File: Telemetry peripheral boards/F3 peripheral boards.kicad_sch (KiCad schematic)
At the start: 37 parts, among them J1 ATS668LSM, J2 1053131108, J3 Potentiometer, J4 Strain Gauge, U1 LM2907M/NOPB, U2 INA125U, U3 MCP2515-I/SO, U4 ISO1050DUB, U5 ATTINY1616-MNR

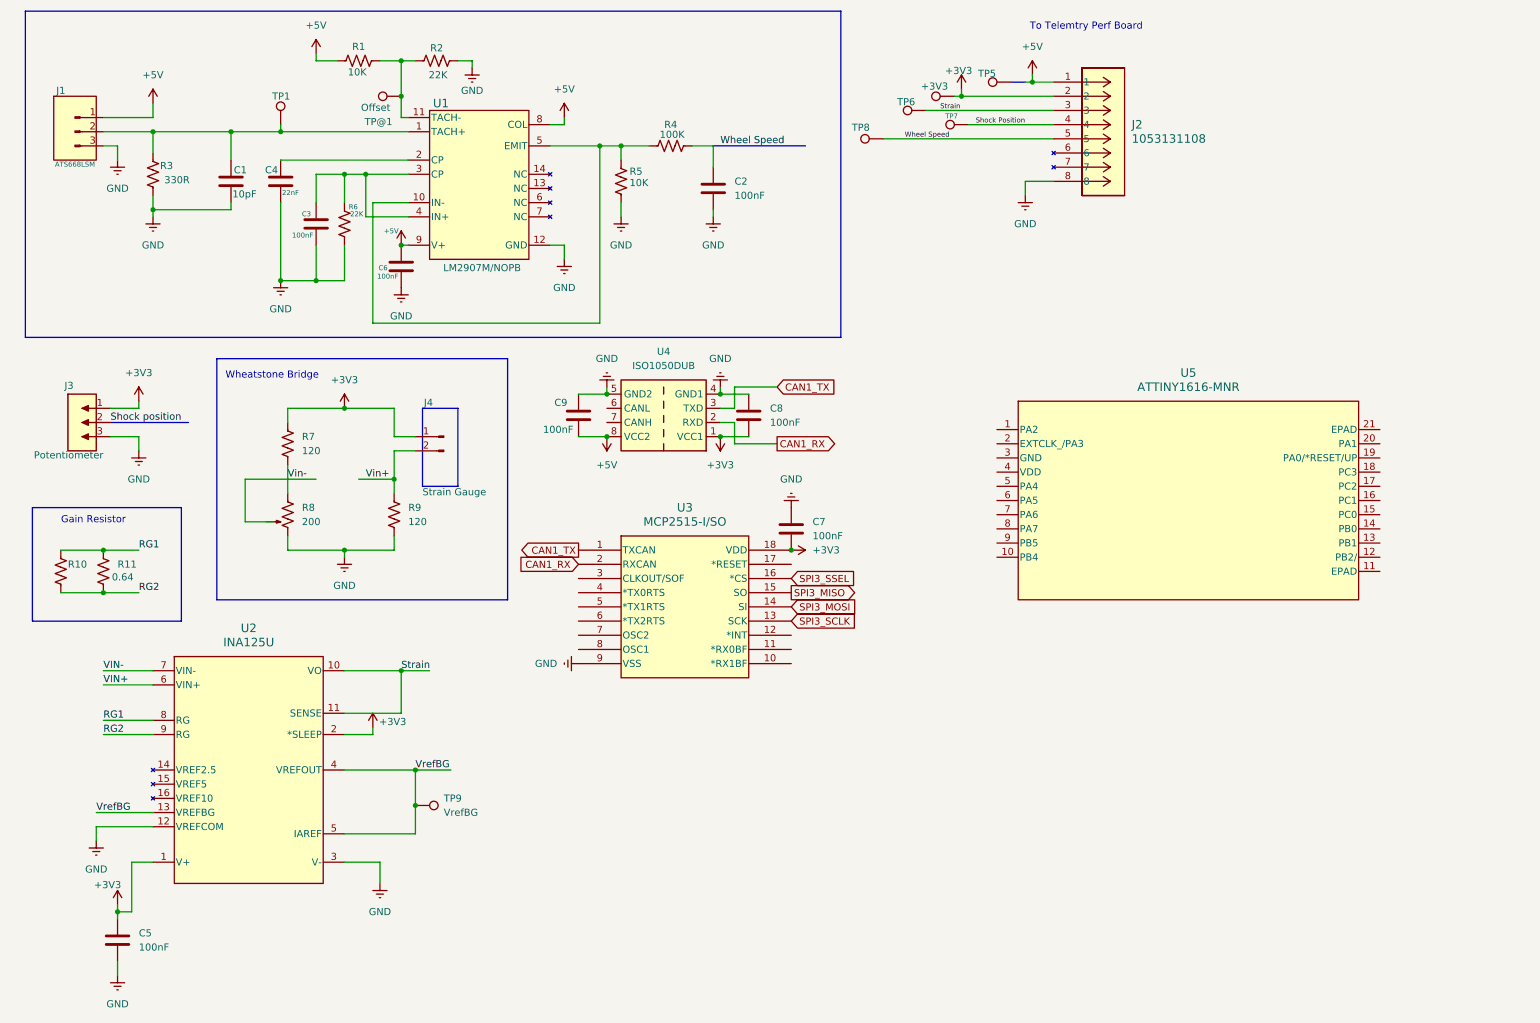
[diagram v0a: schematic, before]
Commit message: Updated peripheral Board
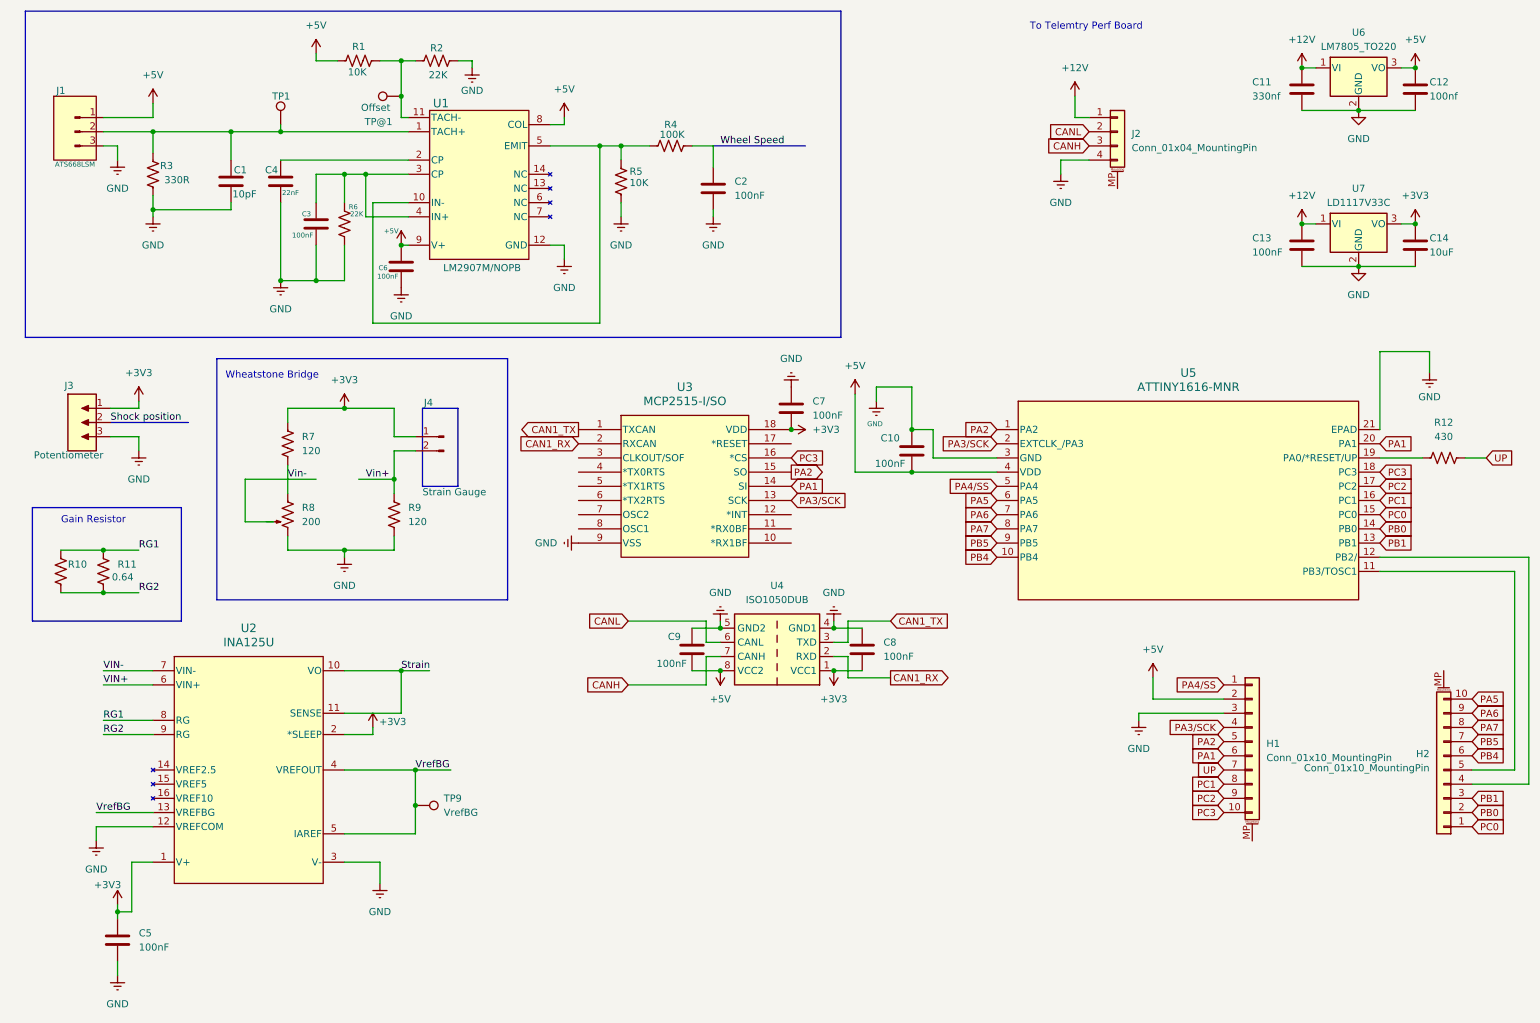
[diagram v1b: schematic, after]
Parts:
- removed +3V3, TP6, TP7, TP8: TestPoint, TestPoint:TestPoint_Loop_D3.80mm_Drill2.0mm, symbol Connector:TestPoint
- removed J2: 1053131108, New Library:CON_1053131108, symbol New_Library:1053131108
- removed TP5: ~, TestPoint:TestPoint_Loop_D3.80mm_Drill2.0mm, symbol Connector:TestPoint
- added C10: 100nF, symbol Device:C
- added C11: 330nf, Capacitor_SMD:C_0805_2012Metric_Pad1.18x1.45mm_HandSolder, symbol Device:C
- added C12: 100nf, Capacitor_SMD:C_0805_2012Metric_Pad1.18x1.45mm_HandSolder, symbol Device:C
- added C13: 100nF, Capacitor_SMD:C_0805_2012Metric_Pad1.18x1.45mm_HandSolder, symbol Device:C
- added C14: 10uF, Capacitor_SMD:C_0805_2012Metric_Pad1.18x1.45mm_HandSolder, symbol Device:C
- added H1, H2: Conn_01x10_MountingPin, symbol Connector_Generic_MountingPin:Conn_01x10_MountingPin
- added J2: Conn_01x04_MountingPin, symbol Connector_Generic_MountingPin:Conn_01x04_MountingPin
- added R12: 430, symbol Device:R_US
- added U6: LM7805_TO220, Package_TO_SOT_THT:TO-220-3_Vertical, symbol Regulator_Linear:LM7805_TO220
- added U7: LD1117V33C, Package_TO_SOT_THT:TO-220-3_Vertical, symbol Regulator_Linear:LM7805_TO220
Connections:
- net SPI3_MISO is gone; now on net PA2: U3.15 (SO)
- net SPI3_MOSI is gone; now on net PA1: U3.14 (SI)
- net SPI3_SCLK is gone; now on net PA3/SCK: U3.13 (SCK)
- net SPI3_SSEL is gone; now on net PC3: U3.16 (*CS)
- net +3V3: now also C14.1, U7.3 (VO)
- net +5V: now also U5.4 (VDD), C10.2, C12.1, H1.2 (Pin_2), U6.3 (VO)
- net GND: now also U5.21 (EPAD), U5.3 (GND), C10.1, C11.2, C12.2, C13.2, C14.2, H1.3 (Pin_3), J2.4 (Pin_4), U6.2 (GND), U7.2 (GND)
- net PA2: now reaches U5.1 (PA2)
- net PA2: now also H1.5 (Pin_5)
- net PB4: now reaches U5.10 (PB4)
- net PB4: now also H2.6 (Pin_6)
- net at U5.11 (PB3/TOSC1): now also H2.5 (Pin_5)
- net at U5.12 (PB2/): now also H2.4 (Pin_4)
- net PB1: now reaches U5.13 (PB1)
- net PB1: now also H2.3 (Pin_3)
- net PB0: now reaches U5.14 (PB0)
- net PB0: now also H2.2 (Pin_2)
- net PC0: now reaches U5.15 (PC0)
- net PC0: now also H2.1 (Pin_1)
- net PC1: now reaches U5.16 (PC1)
- net PC1: now also H1.8 (Pin_8)
- net PC2: now reaches U5.17 (PC2)
- net PC2: now also H1.9 (Pin_9)
- net PC3: now reaches U5.18 (PC3)
- net PC3: now also H1.10 (Pin_10)
- net at U5.19 (PA0/*RESET/UP): now also R12.1
- net PA3/SCK: now reaches U5.2 (EXTCLK_/PA3)
- net PA3/SCK: now also H1.4 (Pin_4)
- net PA1: now reaches U5.20 (PA1)
- net PA1: now also H1.6 (Pin_6)
- net PA4/SS: now reaches U5.5 (PA4)
- net PA4/SS: now also H1.1 (Pin_1)
- net PA5: now reaches U5.6 (PA5)
- net PA5: now also H2.10 (Pin_10)
- net PA6: now reaches U5.7 (PA6)
- net PA6: now also H2.9 (Pin_9)
- net PA7: now reaches U5.8 (PA7)
- net PA7: now also H2.8 (Pin_8)
- net PB5: now reaches U5.9 (PB5)
- net PB5: now also H2.7 (Pin_7)
- net CANL: now reaches U4.6 (CANL)
- net CANL: now also J2.2 (Pin_2)
- net CANH: now reaches U4.7 (CANH)
- net CANH: now also J2.3 (Pin_3)
- new net +12V: C11.1, C13.1, J2.1 (Pin_1), U6.1 (VI), U7.1 (VI)
- new net UP: H1.7 (Pin_7), R12.2
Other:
- moved on the sheet: C7, C8, C9, U3, U4
